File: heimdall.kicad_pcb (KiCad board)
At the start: 2 copper layers, 20 x 32 mm, 15 parts, among them P1 CONN, U1 ESP-01, U2 TLP222A, U3 UA78M33CDCY

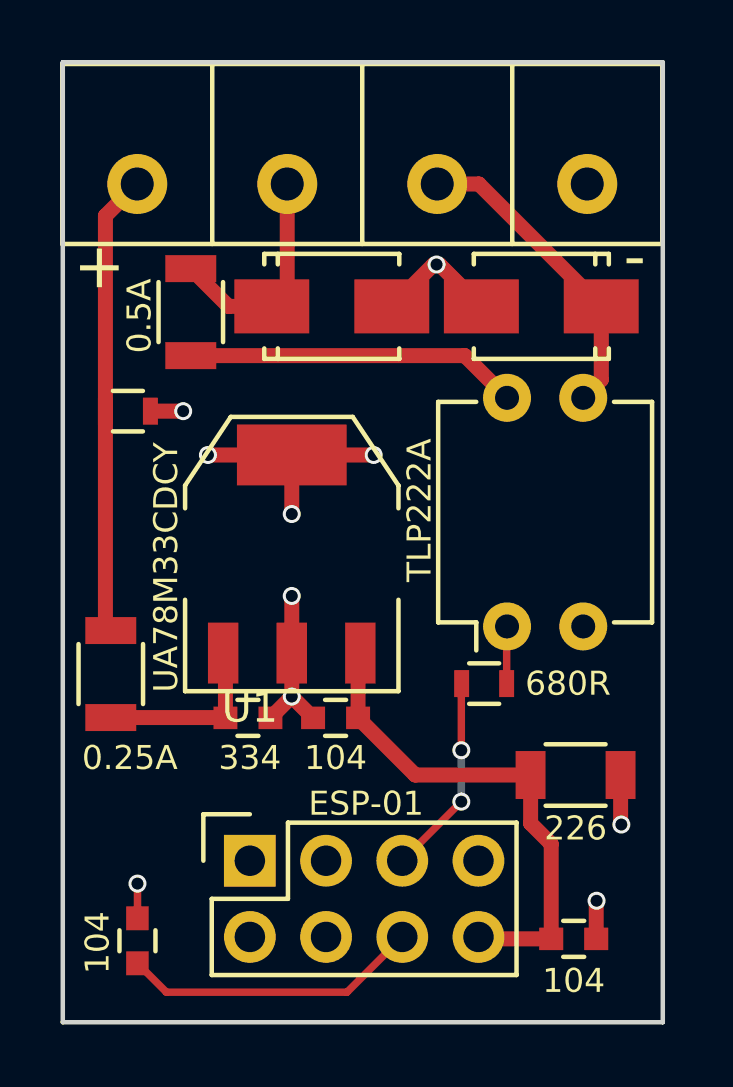
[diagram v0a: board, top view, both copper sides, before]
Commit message: Much faffing, many switch mode supply, very PCB.
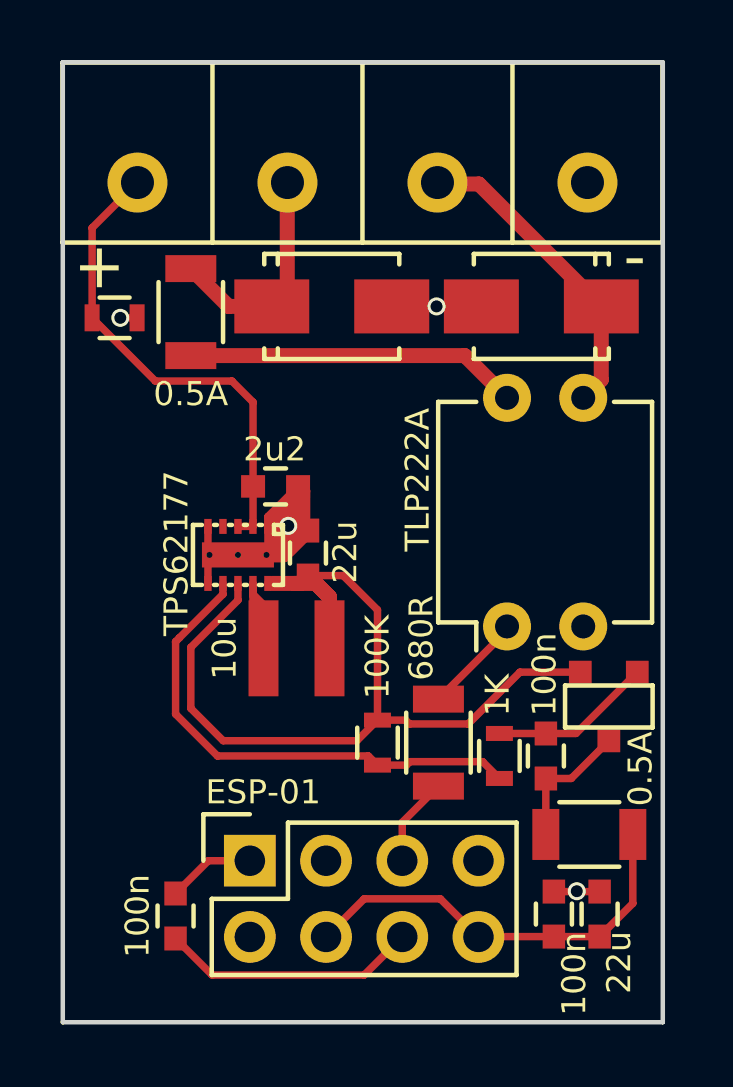
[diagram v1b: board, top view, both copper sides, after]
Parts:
- added C6: 2u2, Capacitors_SMD:C_0603, F.Cu at (107.1, 94.1)
- added L1: 10u, Wurth:WE-TPC, F.Cu at (107.8, 99.5)
- added Q1: FDN304P, Housings_SSOT:SuperSOT-3, F.Cu at (119.2, 100.3)
- added R2: 100K, Resistors_SMD:R_0603, F.Cu at (110.5, 102.7)
- added R3: 1K, Resistors_SMD:R_0603, F.Cu at (114.6, 103.1)
- C1: value 334 -> 22u
- C2, C3, C4: value 104 -> 100n
- C5: value 226 -> 22u; footprint Capacitors_SMD:C_1206 -> Capacitors_SMD:C_0603
- F2: value 0.25A -> 0.5A
- R1: footprint Resistors_SMD:R_0603 -> Resistors_SMD:R_1206
- U1: footprint Socket_Strips:Socket_Strip_Straight_2x04 -> esp:ESP-01-NoSilk
- U3: value UA78M33CDCY -> TPS62177; footprint TO_SOT_Packages_SMD:SOT-223 -> Housing_WSON:WSON-10
- moved F2 16.8 mm to (117.6, 105.7), turned to 180 degrees
- moved P1 7.55 mm to (102.5, 84.0)
- moved C2 7.12 mm to (116.1, 103.1), turned to 90 degrees
- moved C1 5.85 mm to (108.2, 96.4), turned to 90 degrees
- moved C5 4.70 mm to (117.9, 108.4), turned to 90 degrees
- moved U1 4.02 mm to (110.0, 107.9)
- moved D1 3.14 mm to (101.7, 88.5)
- moved R1 2.49 mm to (112.5, 102.7), turned to 270 degrees
- moved C3 1.51 mm to (103.8, 108.5)
- moved U3 1.22 mm to (106.8, 95.5), turned to 270 degrees
- moved C4 1.06 mm to (116.4, 108.4), turned to 90 degrees
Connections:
- C1 pad 1: Net-(C1-Pad1) -> +3V3
- C2 pad 1: +3V3 -> /PWROUT
- C2 pad 2: GND -> Net-(C2-Pad2)
- C4 pad 1: +3V3 -> Net-(C4-Pad1)
- C5 pad 1: +3V3 -> Net-(C4-Pad1)
- D1 pad 1: /VCC_IN -> /VCC
- F2 pad 1: /VCC_IN -> Net-(C4-Pad1)
- F2 pad 2: Net-(C1-Pad1) -> /PWROUT
- P1 pad 1: /VCC_IN -> /VCC
- U1 pad 2: Net-(U1-Pad2) -> (no net)
- U1 pad 3: Net-(U1-Pad3) -> (no net)
- U1 pad 4: Net-(U1-Pad4) -> Net-(C4-Pad1)
- U1 pad 7: Net-(U1-Pad7) -> (no net)
- U1 pad 8: +3V3 -> Net-(C4-Pad1)
- U3 pad 1: Net-(C1-Pad1) -> GND
- U3 pad 2: GND -> /VCC
- U3 pad 3: +3V3 -> /VCC
- U3 pad 4: GND -> (no net)
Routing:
- net /PG: track 0.00 -> 16.8 mm
- net /VCC: track 0.00 -> 16.5 mm
- net +3V3: track 17.0 -> 33.4 mm
- net /VCC_IN: track 15.8 -> 0.00 mm
- net Net-(C4-Pad1): track 0.00 -> 14.0 mm
- net Net-(L1-Pad1): track 0.00 -> 6.93 mm
- net Net-(C1-Pad1): track 6.02 -> 0.00 mm
- net Net-(C2-Pad2): track 0.00 -> 5.44 mm
- net GND: track 22.2 -> 26.8 mm, vias 10 -> 4
- net /PWROUT: track 0.00 -> 4.48 mm
- net /RELAY_TRIGGER: track 6.82 -> 3.51 mm, vias 2 -> 0
- net Net-(R1-Pad1): track 1.91 -> 3.39 mm
- net Net-(C3-Pad1): track 9.90 -> 8.59 mm
- removed copper zone on F.Cu, net GND
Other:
- board text added: "Hark <pcb@harkonen.net> Heimdall V1 08/06/16 http://github.com/HarkonenBade/heimdall"
- board text removed: "Hark <pcb@harkonen.net> Heimdall V1 18/05/16 https://goo.gl/4EXW3O"
